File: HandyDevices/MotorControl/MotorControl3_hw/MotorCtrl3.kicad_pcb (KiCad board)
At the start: 2 copper layers, 90 x 108 mm, 279 parts, among them Q1 USBLC6_2XX, Q10 BC817, Q11 BC817, Q12 BC817, Q13 IRF7425, Q14 IRF7425, Q2 MMBT2222, Q3 IRLML9303, Q4 MMBT2222, Q5 IRLML9303, Q6 MMBT2222, Q7 IRLML9303, Q8 MMBT2222, Q9 BC817, SW1 BUTTON, U1 L6470, U2 L6470, U3 L6470, U4 L6470

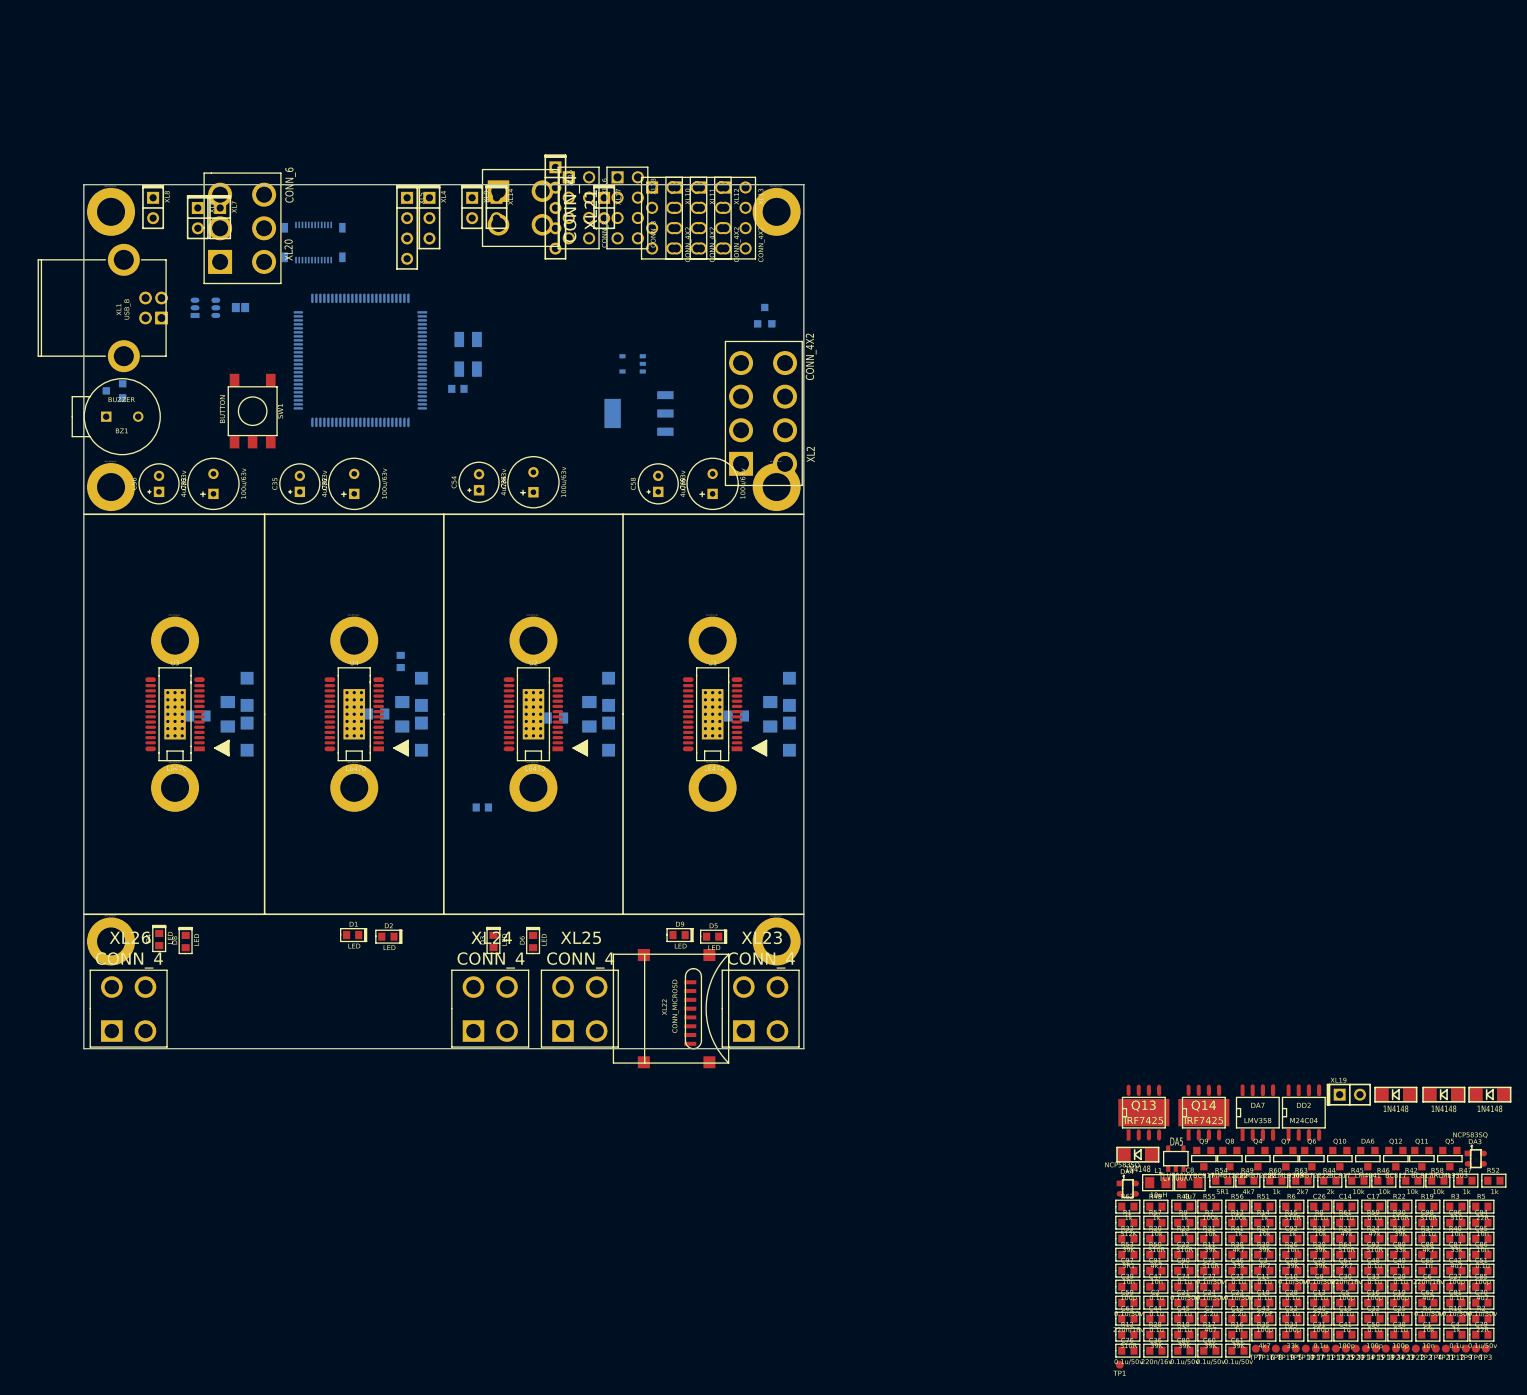
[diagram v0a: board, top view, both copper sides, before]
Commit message: MotorCtrl3 start to trace board.
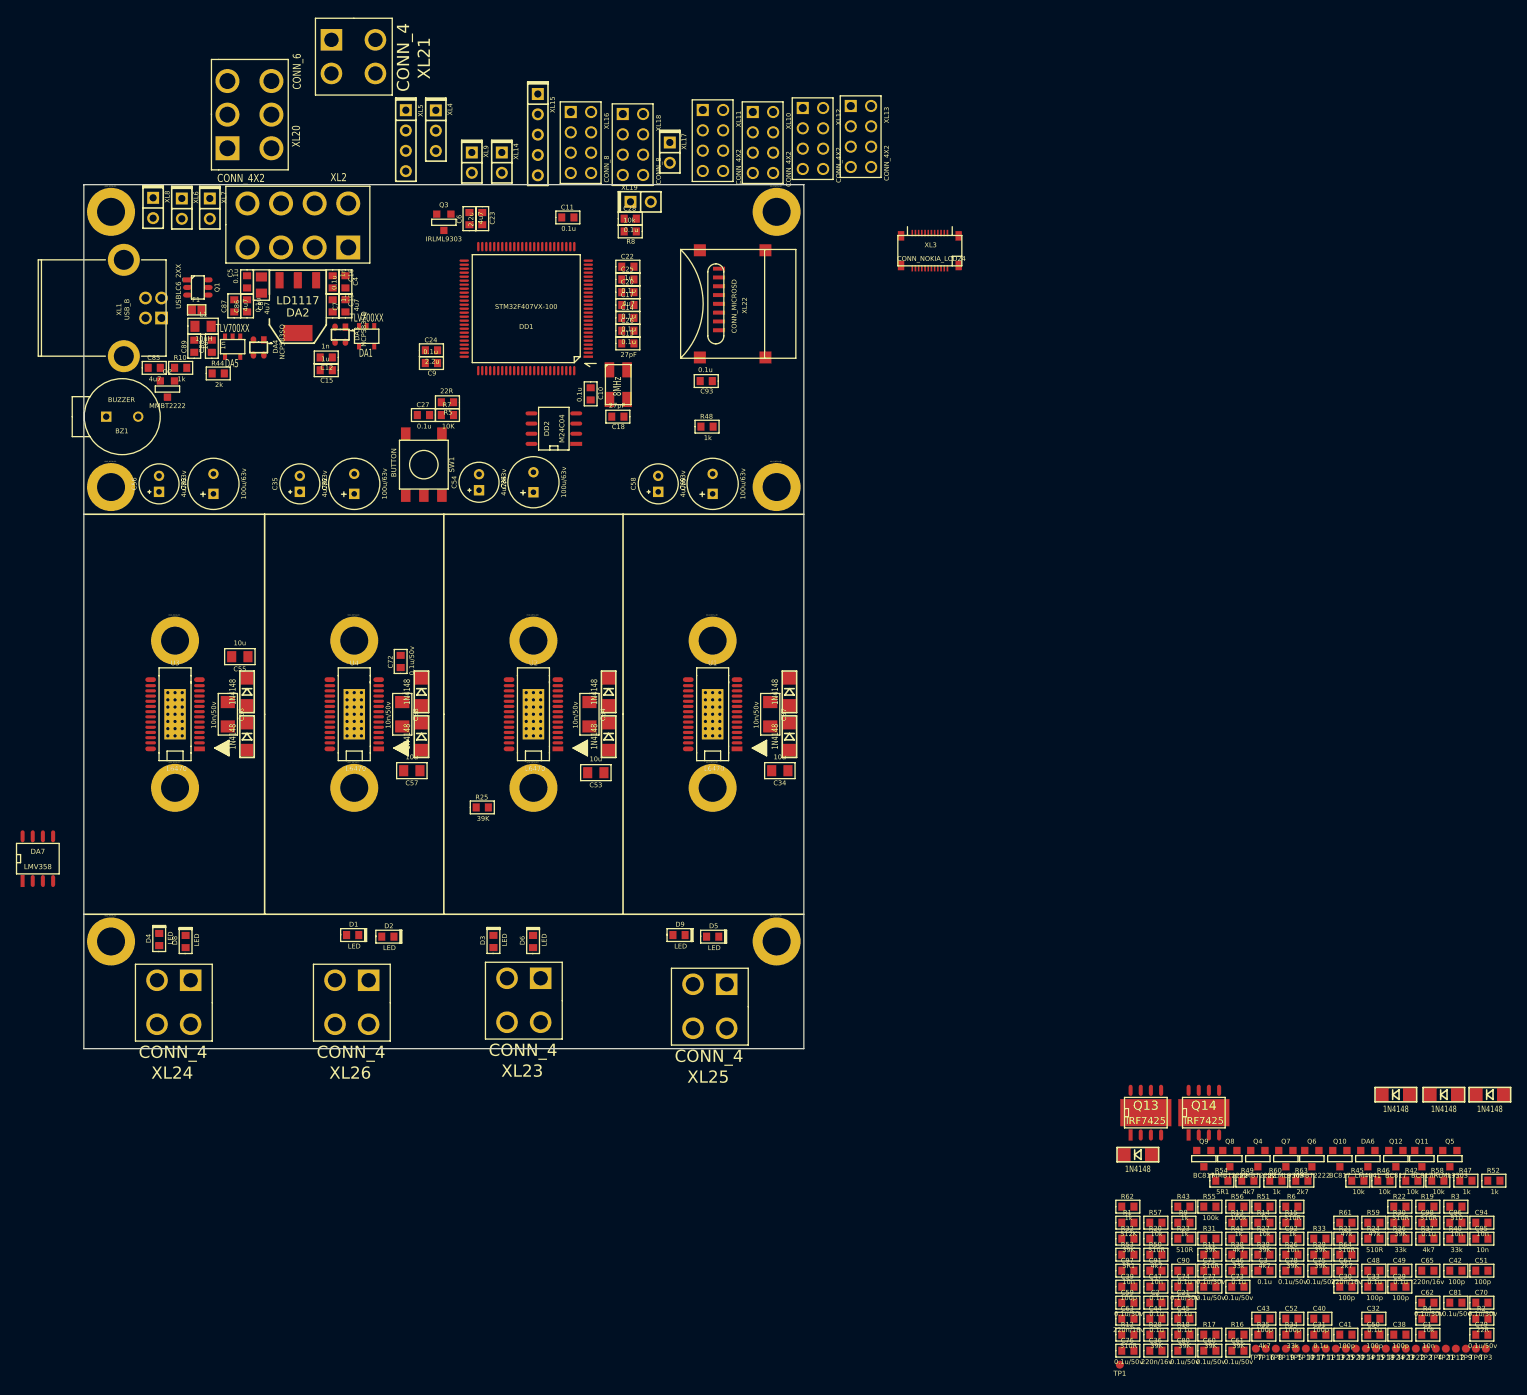
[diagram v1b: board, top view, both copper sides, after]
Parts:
- C20, C34, C37, C53, C55, C57, C64, C66, C68, C72, D10, D11, D12, D13, D14, D15, D16, D7, DA1, DA2, DD1, F1, Q1, Q2, Q3, R25, XL3, XTAL1: moved to F.Cu
- moved C85 201.8 mm to (184.8, 109.9)
- moved R10 198.8 mm to (188.1, 109.9)
- moved C86 194.7 mm to (196.4, 102.2), turned to 90 degrees
- moved C87 193.3 mm to (194.8, 102.2), turned to 90 degrees
- moved C4 191.3 mm to (208.7, 99.2), turned to 270 degrees
- moved C88 189.7 mm to (192.0, 107.2), turned to 90 degrees
- moved C89 188.7 mm to (189.8, 107.2), turned to 90 degrees
- moved C5 187.5 mm to (196.4, 99.2), turned to 270 degrees
- moved C19 182.5 mm to (207.1, 102.2), turned to 90 degrees
- moved C16 182.3 mm to (207.1, 99.2), turned to 270 degrees
- moved C6 179.4 mm to (224.2, 91.2), turned to 90 degrees
- moved DA3 175.4 mm to (208.1, 105.8), turned to 270 degrees
- moved C15 174.1 mm to (206.3, 110.2), turned to 180 degrees
- moved R44 171.7 mm to (192.8, 110.6)
- moved C27 168.9 mm to (218.4, 115.8)
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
